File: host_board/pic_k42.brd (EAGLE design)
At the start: 54.6 x 77.5 mm, 54 parts, among them IC1 PIC18F57K42-E_PT, IC2 REF3440IDBVR, IC3 MAX232, IC4 ILAMP, K1 G6K-2P, Q1 ASF1, X1 RX-2, X2 TX-2, X3 RESETJMP, X5 PORTA, X6 PORTD, X7 PORTB

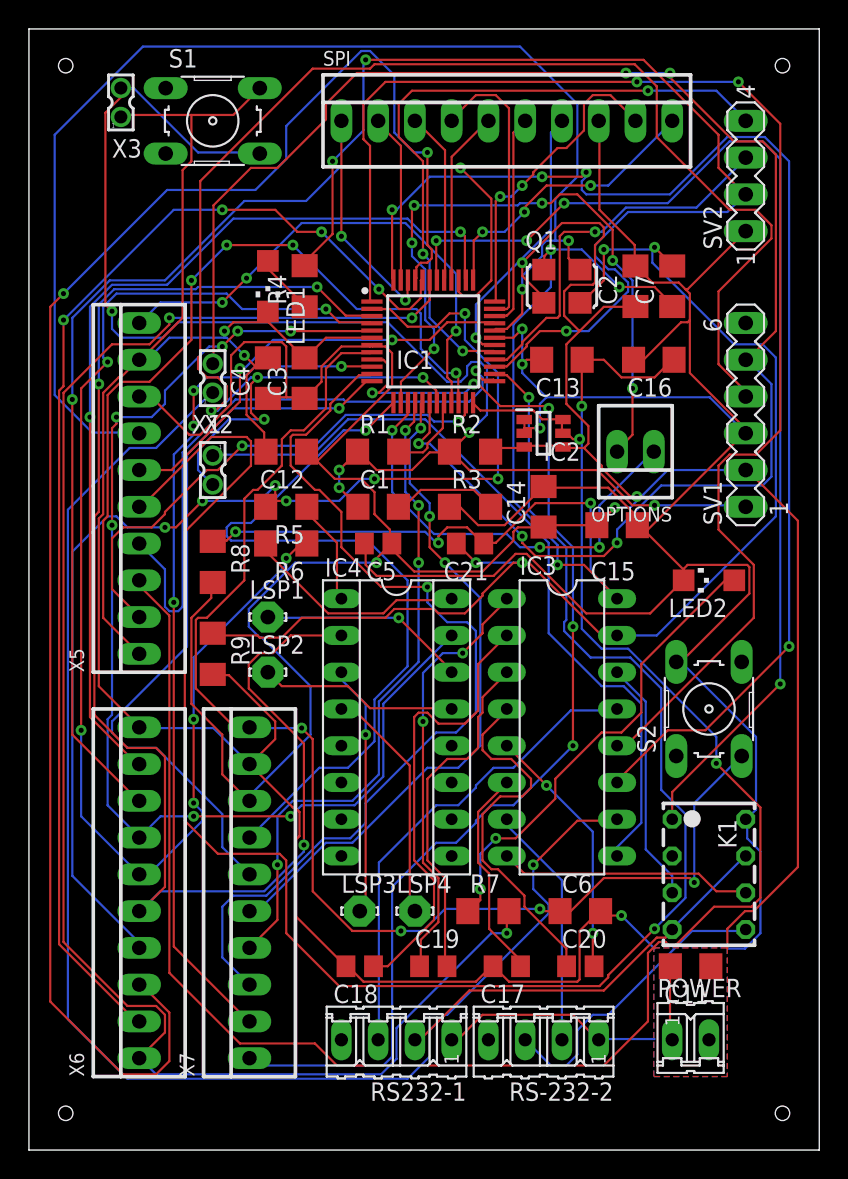
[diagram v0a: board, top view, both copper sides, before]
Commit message: update
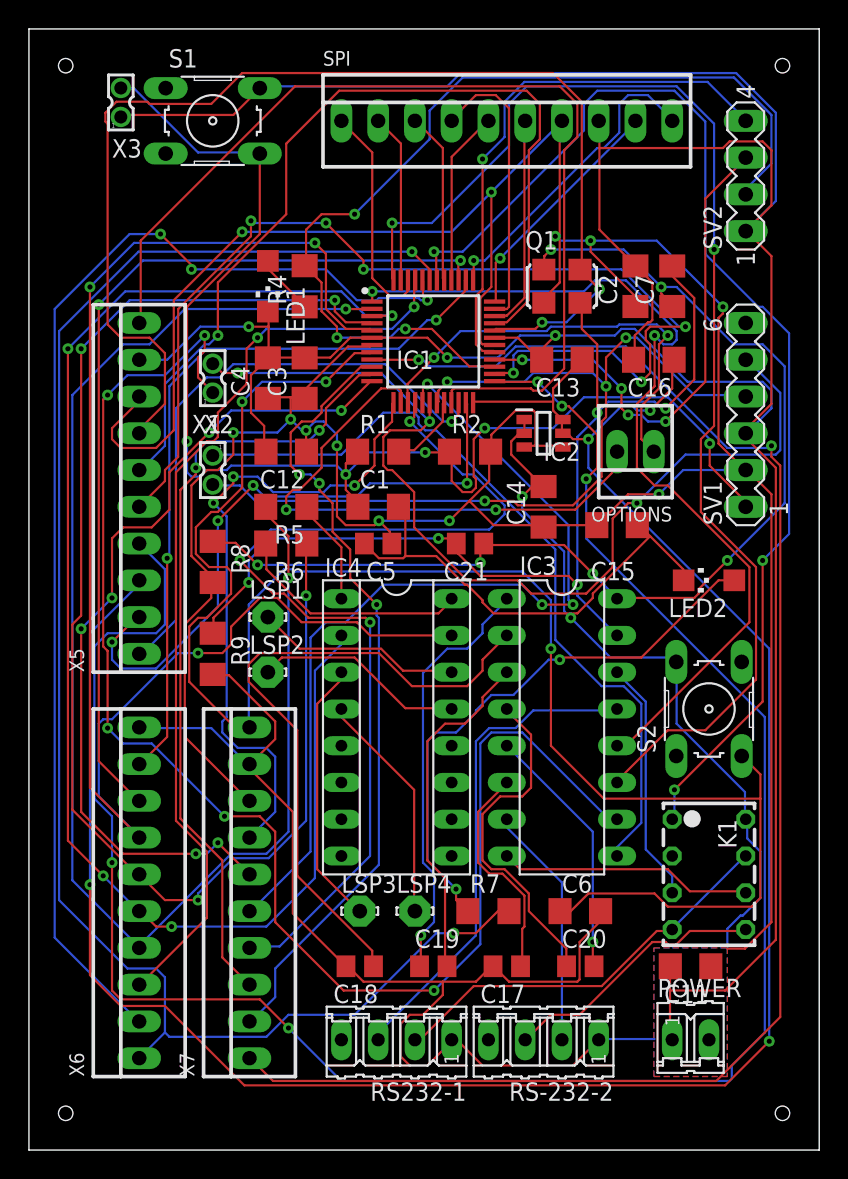
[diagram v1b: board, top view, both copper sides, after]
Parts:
- removed R3: 0, rcl:R1206
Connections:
- removed net N$3: C1.2, R3.2
- net VSS: now also C1.2; no longer R3.1
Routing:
- net N$36: track 43.0 -> 141.1 mm, vias 1 -> 5
- net VSS: track 335.6 -> 396.6 mm, vias 6 -> 5
- net N$35: track 126.7 -> 75.5 mm, vias 2 -> 6
- net N$45: track 114.6 -> 63.8 mm
- net N$6: track 111.1 -> 61.9 mm
- net N$7: track 114.5 -> 69.4 mm, vias 5 -> 3
- net N$39: track 35.5 -> 68.9 mm, vias 3 -> 0
- net N$40: track 30.2 -> 63.3 mm, vias 2 -> 1
- net N$18: track 95.6 -> 62.8 mm
- net N$43: track 90.0 -> 122.7 mm, vias 4 -> 3
- net N$53: track 79.7 -> 110.2 mm, vias 5 -> 2
- net N$56: track 45.6 -> 68.5 mm, vias 4 -> 3
- net N$49: track 81.2 -> 103.7 mm, vias 7 -> 3
- net VDD: track 228.2 -> 246.8 mm, vias 5 -> 12
- net N$46: track 84.2 -> 100.0 mm, vias 7 -> 2
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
